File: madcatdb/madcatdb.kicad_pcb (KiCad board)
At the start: 2 copper layers, 46 x 11 mm, 11 parts, among them J1 USB_C_Receptacle_USB2.0, J2 Conn_01x04, U1 USBLC6-2SC6

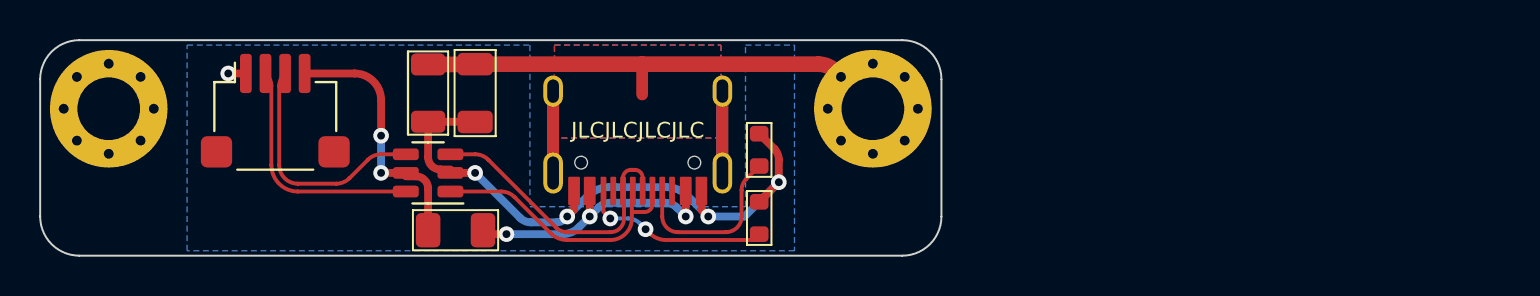
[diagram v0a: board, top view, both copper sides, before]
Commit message: generated prod files
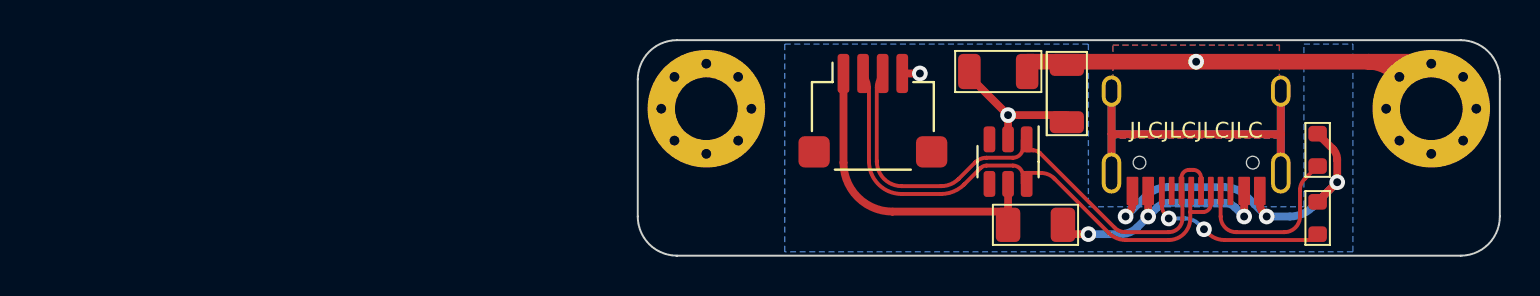
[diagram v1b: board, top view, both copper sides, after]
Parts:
- added H3: JLCJLCJLCJLC, Crokto:JLCJLCJLCJLC, F.Cu at (84.5, 4.60)
- added H3: JLCJLCJLCJLC, Crokto:JLCJLCJLCJLC, F.Cu at (28.5, 19.1)
- H3: value jlc -> JLCJLCJLCJLC
- U1: value USBLC6-2SC6 -> SRV05-4
- moved R3 32.6 mm to (21.9, 2.73)
- moved H1 30.5 mm to (3.50, 3.50)
- moved J2 30.5 mm to (12.0, 3.92)
- moved U1 29.6 mm to (18.9, 6.20), turned to -90 degrees
- moved F1 29.6 mm to (20.3, 9.43)
- moved J1 28.7 mm to (28.5, 3.65), turned to 180 degrees
- moved R1 28.5 mm to (34.7, 5.60)
- moved R2 28.5 mm to (34.7, 9.07)
- moved H2 28.5 mm to (40.5, 3.50)
- moved H3 28.5 mm to (28.5, 4.60)
- moved C1 26.7 mm to (18.4, 1.60), turned to 0 degrees
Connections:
- J1 pad A6: DB+ -> D+
- J1 pad A7: DB- -> D-
- J1 pad B6: DB+ -> D+
- J1 pad B7: DB- -> D-
- J2 pad 1: GND -> +5V
- J2 pad 4: +5V -> GND
- U1 pad 1: DB- -> D+
- U1 pad 3: DB+ -> unconnected-(U1-Pad3)
- U1 pad 4: D+ -> unconnected-(U1-Pad4)
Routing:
- net Earth: track 41.9 -> 58.8 mm, vias 0 -> 1
- net D+: track 12.3 -> 28.1 mm
- net D-: track 12.3 -> 28.1 mm
- net DB+: track 15.0 -> 0.00 mm
- net DB-: track 14.1 -> 0.00 mm
- net GND: track 33.4 -> 27.7 mm
- net +5V: track 13.2 -> 16.4 mm, vias 2 -> 0
- net VBUS: track 13.8 -> 12.8 mm
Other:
- board size 46 x 11 mm -> 44 x 11 mm
